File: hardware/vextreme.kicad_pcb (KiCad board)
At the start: 2 copper layers, 48 x 66.1 mm, 63 parts, among them CON1 vectrex-edge-connector, J1 USB_C_Receptacle_USB2.0, J2 Conn_01x04_Male, J3 Conn_01x03_Male, J4 FTSH-105-01-F-DV-K, SW1 TS-1002S-12026C, SW2 TS-1002S-12026C, U1 LM1117-3.3, U2 STM32F411RCTx, U3 74LVC1G32, U4 SN74LVC8T245DB, U5 W25Q128, U6 TPD4E02B04DQA, Y1 8MHz

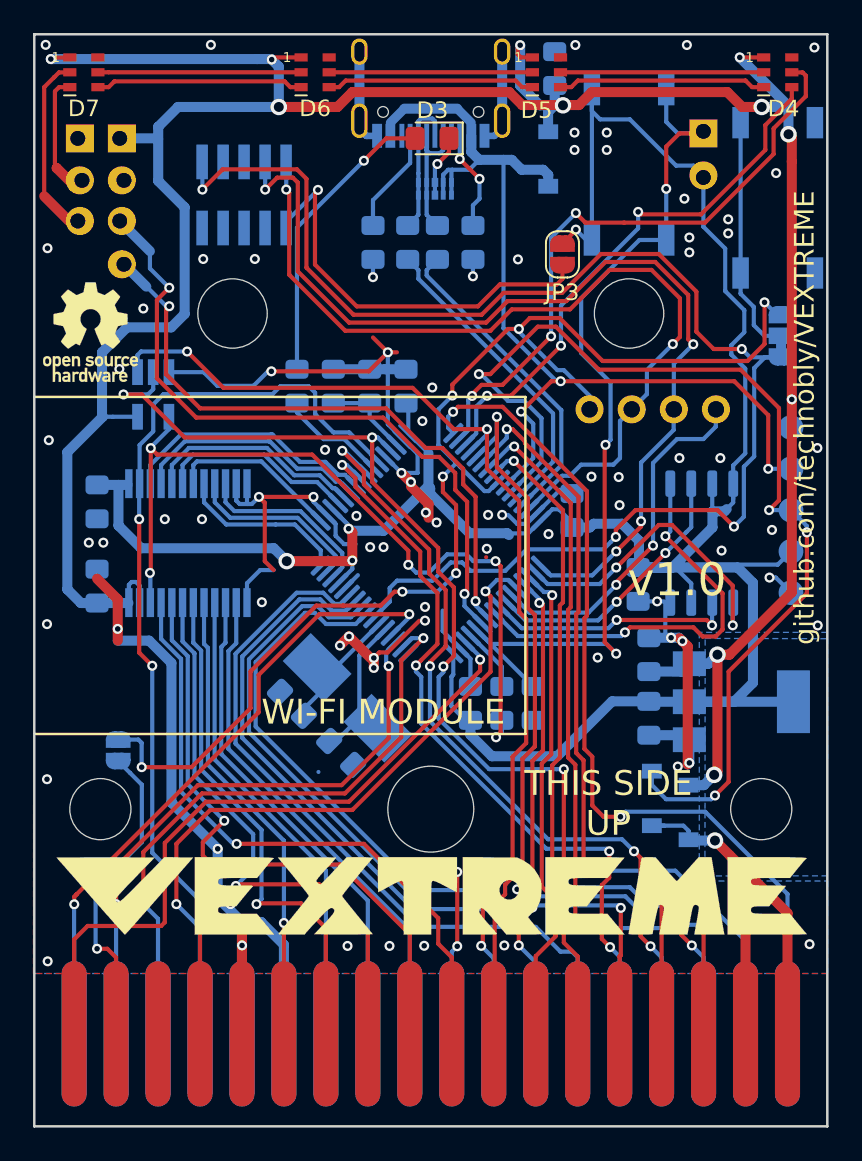
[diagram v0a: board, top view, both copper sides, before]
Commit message: Migrate hardware to KiCad 10
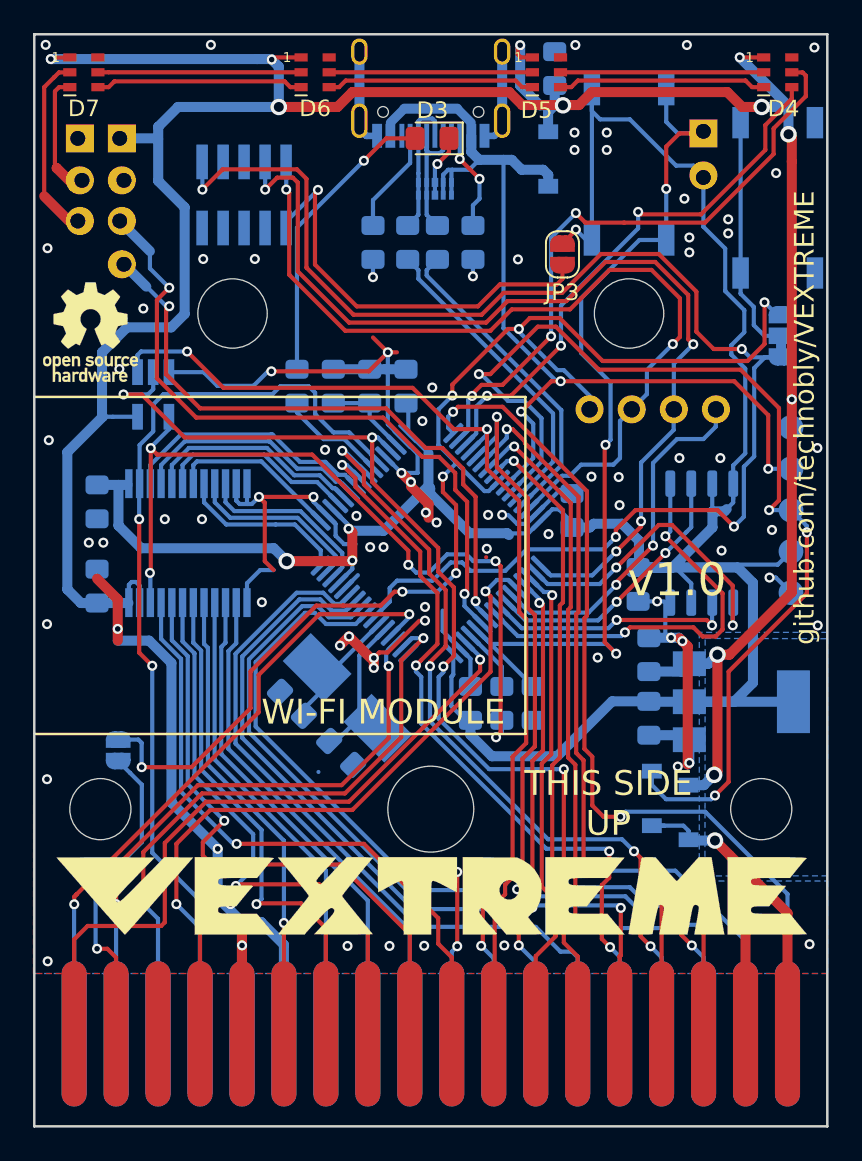
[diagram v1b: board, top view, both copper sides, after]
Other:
- net class Default removed
- net class Large removed
